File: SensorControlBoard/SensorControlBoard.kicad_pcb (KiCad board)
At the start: 2 copper layers, 79 parts, among them J1 Micro_SD_Card, J10 Conn_01x05_Pin, J11 USB_C_Receptacle_USB2.0, J2 Conn_01x02_Pin, J3 Conn_02x10_Odd_Even, J4 Conn_01x10_Pin, J5 Conn_01x10_Pin, J6 Conn_01x02_Pin, J7 Conn_01x02_Pin, J8 Conn_01x02_Pin, SW1 SW_SPDT, U1 STM32F103C8T6TR, U10 ASMB-TTF0-0A20B, U11 ASMB-TTF0-0A20B, U12 AT24CS04-XHM, U13 OPT3002DNPR, U2 TLV1117LV33DCYR, U3 TMAG5273B1QDBVR, U4 TMAG5170-Q1, U5 LP5018RSMR, U6 ASMB-TTF0-0A20B, U7 ASMB-TTF0-0A20B, U8 ASMB-TTF0-0A20B, U9 ASMB-TTF0-0A20B, Y1 16MHz OSC

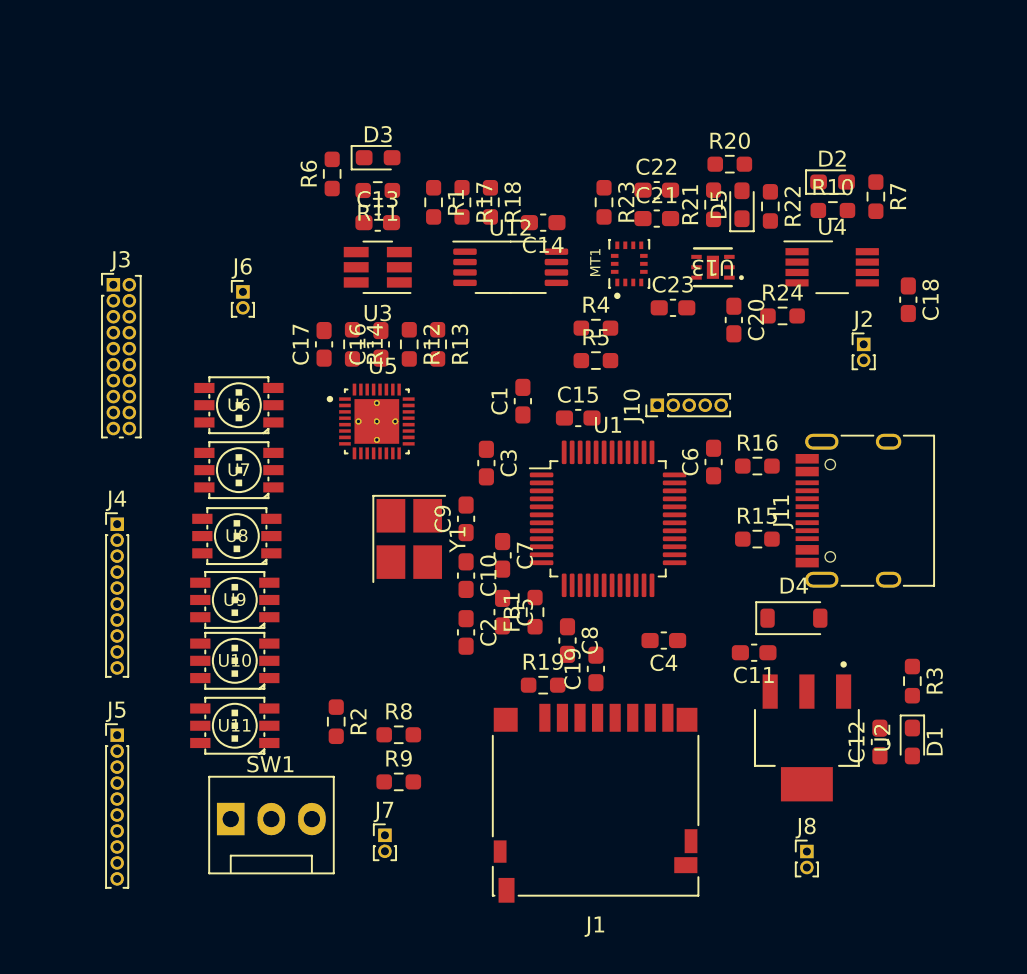
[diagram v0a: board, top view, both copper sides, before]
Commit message: Initial Routing finished
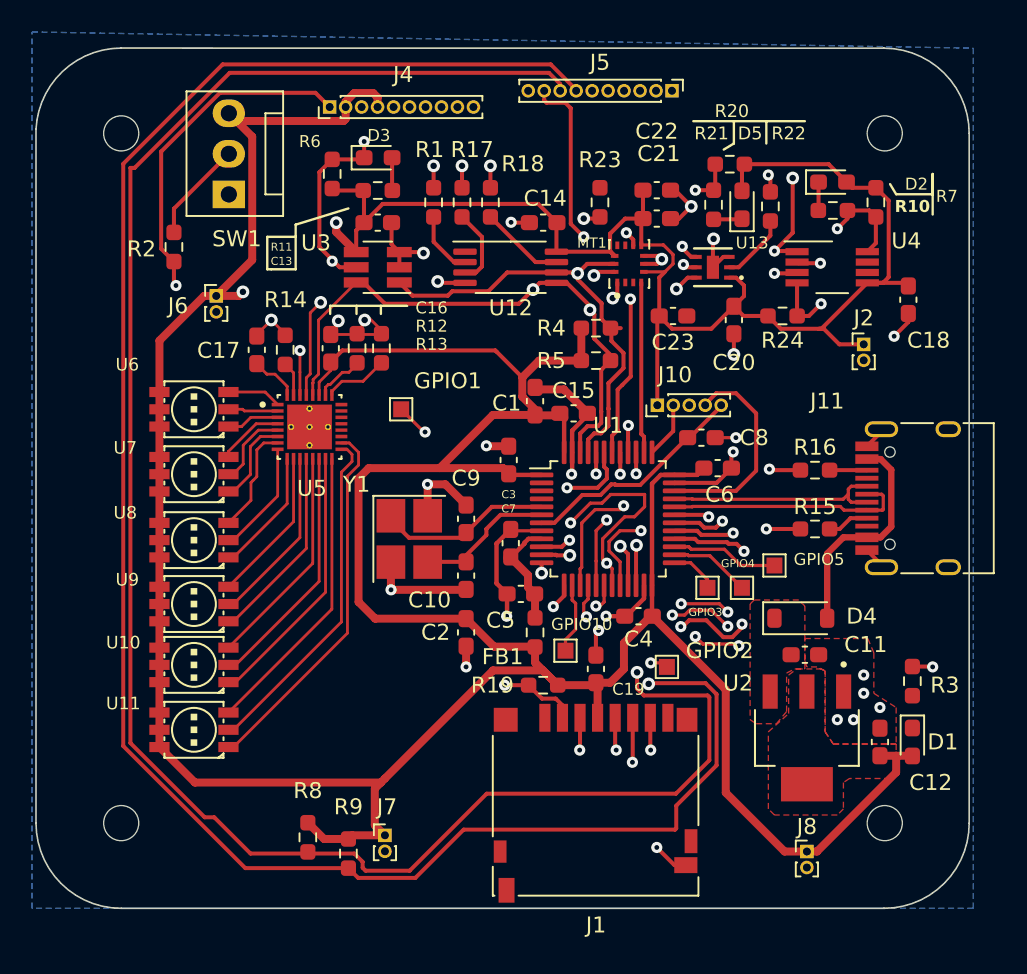
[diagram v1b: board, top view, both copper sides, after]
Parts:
- removed J3: Conn_02x10_Odd_Even, Connector_PinHeader_1.00mm:PinHeader_2x10_P1.00mm_Vertical
- added GPIO1: TestPoint, TestPoint:TestPoint_Pad_1.0x1.0mm, F.Cu at (91.2, 46.5)
- added GPIO10: TestPoint, TestPoint:TestPoint_Pad_1.0x1.0mm, F.Cu at (101.5, 61.6)
- added GPIO2: TestPoint, TestPoint:TestPoint_Pad_1.0x1.0mm, F.Cu at (107.8, 62.6)
- added GPIO3: TestPoint, TestPoint:TestPoint_Pad_1.0x1.0mm, F.Cu at (110.4, 57.7)
- added GPIO4: TestPoint, TestPoint:TestPoint_Pad_1.0x1.0mm, F.Cu at (112.5, 57.7)
- added GPIO5: TestPoint, TestPoint:TestPoint_Pad_1.0x1.0mm, F.Cu at (114.6, 56.3)
- added H1: MountingHole, MountingHole:MountingHole_2.2mm_M2, F.Cu at (121.5, 29.2)
- added H2: MountingHole, MountingHole:MountingHole_2.2mm_M2, F.Cu at (73.7, 29.2)
- added H3: MountingHole, MountingHole:MountingHole_2.2mm_M2, F.Cu at (73.7, 72.4)
- added H4: MountingHole, MountingHole:MountingHole_2.2mm_M2, F.Cu at (121.5, 72.4)
- moved J5 53.2 mm to (108.1, 26.5), turned to -90 degrees
- moved SW1 39.1 mm to (80.4, 33.0), turned to 90 degrees
- moved R2 31.4 mm to (77.0, 36.3), turned to 90 degrees
- moved J4 29.3 mm to (86.7, 27.6), turned to 90 degrees
- moved C8 15.2 mm to (110.0, 48.3), turned to 0 degrees
- moved R8 8.58 mm to (85.3, 73.3), turned to -90 degrees
- moved R9 5.48 mm to (87.9, 74.3), turned to -90 degrees
- moved C17 4.23 mm to (82.1, 42.8)
- moved R14 4.23 mm to (83.9, 42.8)
- moved U5 4.23 mm to (85.4, 47.6)
- moved J11 3.82 mm to (124.4, 52.0)
- moved R15 3.66 mm to (117.1, 54.0)
- moved R16 3.62 mm to (117.1, 50.3)
- moved R13 3.53 mm to (90.0, 42.7)
- moved R12 3.28 mm to (88.4, 42.7)
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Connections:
- D3 pad 1: GPIO_4 -> GPIO_7
- J1 pad 2: GPIO_5 -> GPIO_9
- J4 pad 1: /uController/GPIO_11 -> /uController/BOOT0
- J4 pad 10: SPI1_SCK -> /uController/ADC1_0
- J4 pad 2: /uController/GPIO_12 -> +3.3V
- J4 pad 3: /uController/GPIO_13 -> GND
- J4 pad 4: /uController/GPIO_14 -> +3.3V
- J4 pad 5: /uController/ADC1_0 -> GND
- J4 pad 6: /uController/ADC1_7 -> /uController/ADC2_6
- J4 pad 7: /uController/ADC1_8 -> /uController/ADC1_7
- J4 pad 8: /uController/ADC2_5 -> /uController/ADC1_8
- J4 pad 9: /uController/ADC2_6 -> /uController/ADC2_5
- J5 pad 10: /uController/BOOT0 -> /uController/UART1_RX
- J5 pad 3: /uController/UART1_TX -> SPI1_SCK
- J5 pad 4: /uController/UART1_RX -> unconnected-(J5-Pin_4-Pad4)
- J5 pad 9: /uController/NRST -> /uController/UART1_TX
- MT1 pad 4: GPIO_7 -> GPIO_14
- MT1 pad 9: GPIO_8 -> GPIO_13
- R10 pad 2: GPIO_2 -> GPIO_6
- R19 pad 2: GPIO_5 -> GPIO_9
- R20 pad 1: GPIO_6 -> GPIO_12
- R21 pad 2: GPIO_6 -> GPIO_12
- R24 pad 2: GPIO_1 -> GPIO_11
- R6 pad 2: GPIO_4 -> GPIO_7
- R7 pad 2: GPIO_2 -> GPIO_6
- U1 pad 11: /uController/GPIO_7 -> GPIO_7
- U1 pad 12: /uController/GPIO_8 -> GPIO_8
- U1 pad 13: /uController/GPIO_9 -> GPIO_9
- U1 pad 14: /uController/GPIO_10 -> GPIO_10
- U1 pad 25: /uController/GPIO_3 -> GPIO_3
- U1 pad 26: /uController/GPIO_4 -> GPIO_4
- U1 pad 27: /uController/GPIO_5 -> GPIO_5
- U1 pad 28: /uController/GPIO_6 -> GPIO_6
- U1 pad 29: /uController/GPIO_11 -> GPIO_11
- U1 pad 30: /uController/GPIO_12 -> GPIO_12
- U1 pad 31: /uController/GPIO_13 -> GPIO_13
- U1 pad 38: /uController/GPIO_14 -> GPIO_14
- U13 pad 5: GPIO_6 -> GPIO_12
- U3 pad 5: GPIO_4 -> GPIO_7
- U4 pad 4: GPIO_1 -> GPIO_11
- U4 pad 8: GPIO_2 -> GPIO_6
- U5 pad 30: GPIO_3 -> GPIO_8
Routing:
- net +3.3V: track 0.00 -> 316.0 mm, vias 0 -> 2
- net /uController/I2C2_SCL: track 0.00 -> 134.1 mm, vias 0 -> 2
- net /uController/I2C2_SDA: track 0.00 -> 128.9 mm, vias 0 -> 2
- net /uController/ADC1_7: track 0.00 -> 126.9 mm, vias 0 -> 3
- net SPI1_SCK: track 0.00 -> 115.7 mm, vias 0 -> 4
- net SPI1_MOSI: track 0.00 -> 96.4 mm, vias 0 -> 3
- net GND: track 0.00 -> 90.3 mm, vias 0 -> 35
- net /uController/ADC2_6: track 0.00 -> 87.7 mm, vias 0 -> 3
- net SPI1_MISO: track 0.00 -> 87.2 mm, vias 0 -> 3
- net /uController/ADC1_8: track 0.00 -> 84.2 mm, vias 0 -> 3
- net /uController/ADC2_5: track 0.00 -> 82.0 mm, vias 0 -> 3
- net I2C1_SCL: track 0.00 -> 74.4 mm, vias 0 -> 3
- net /uController/BOOT0: track 0.00 -> 63.7 mm, vias 0 -> 2
- net I2C1_SDA: track 0.00 -> 61.6 mm, vias 0 -> 4
- net /uController/UART1_RX: track 0.00 -> 48.1 mm, vias 0 -> 1
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- added copper zone on F.Cu, net +3.3V
- added copper zone on B.Cu, net GND
- added copper zone on F.Cu, net GND
- added copper zone on F.Cu, net VBUS
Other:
- board outline added: 58.4 x 53.9 mm
- copper layers 2 -> 4
